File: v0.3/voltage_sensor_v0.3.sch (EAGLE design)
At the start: 56 parts, among them IC1 AP2112K-3.3TRG1, J2 236-404_000-009_999-950, J3 MC000048, J9 RJ11-6, T1 ZMPT101B, T2 ZMPT101B, T3 ZMPT101B

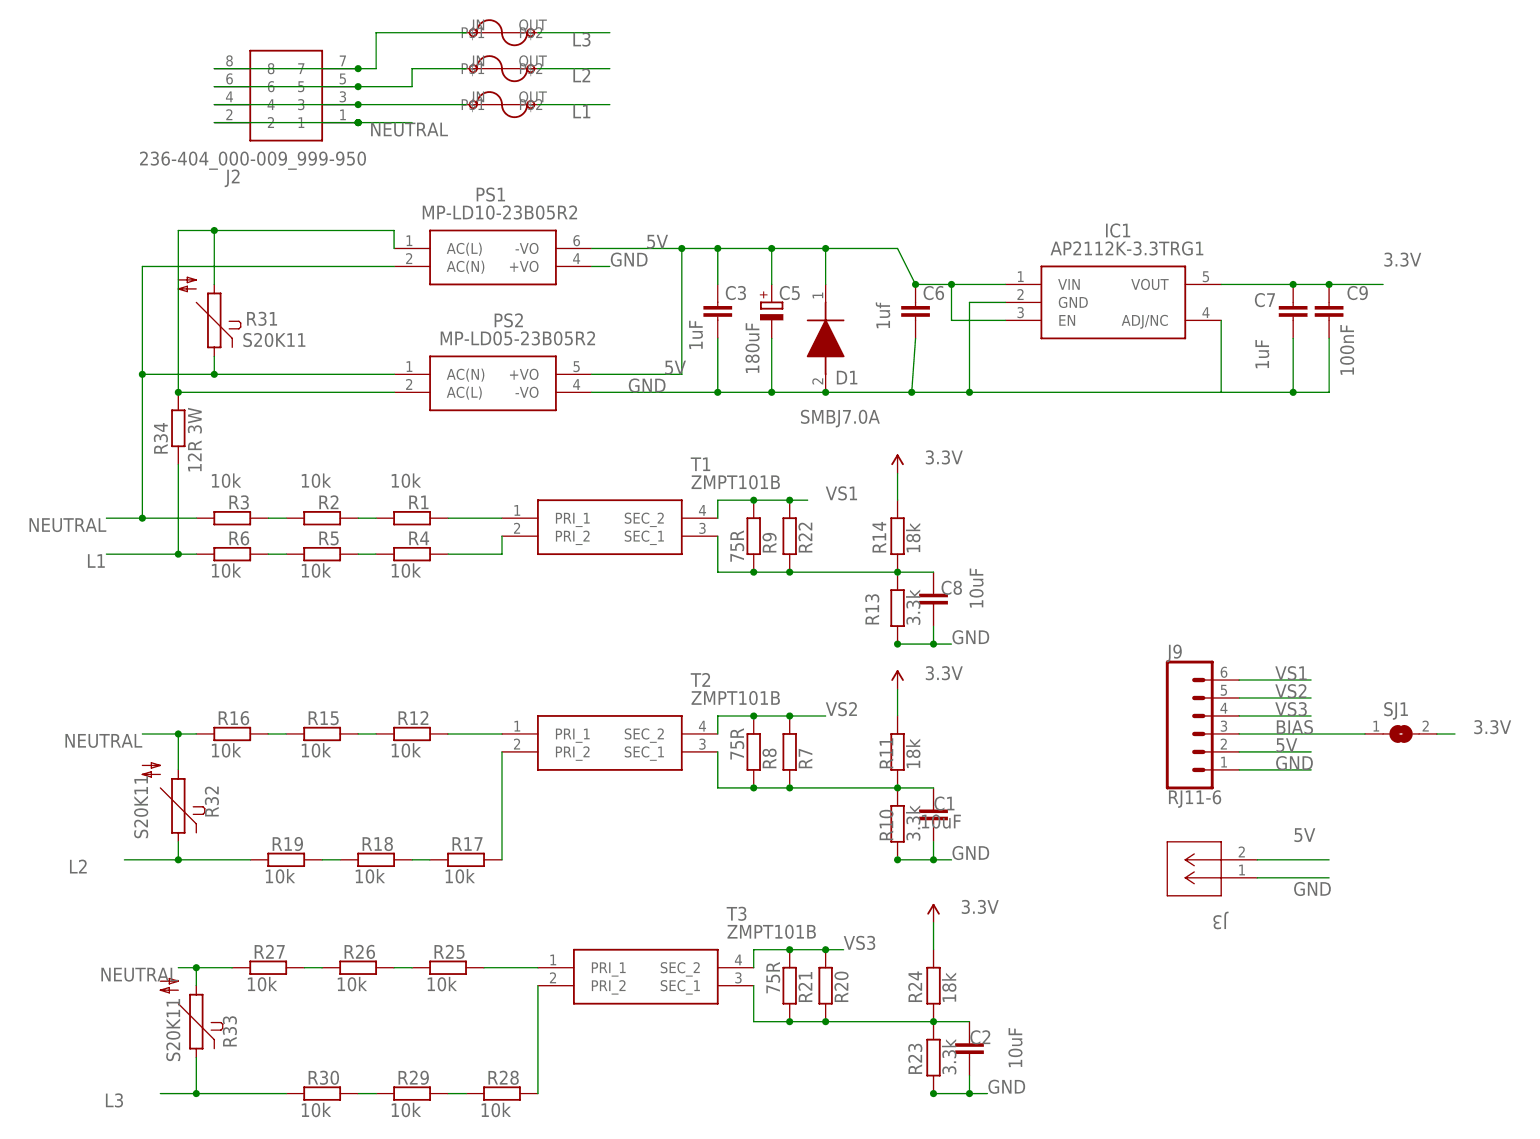
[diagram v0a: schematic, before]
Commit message: v0.3 changes
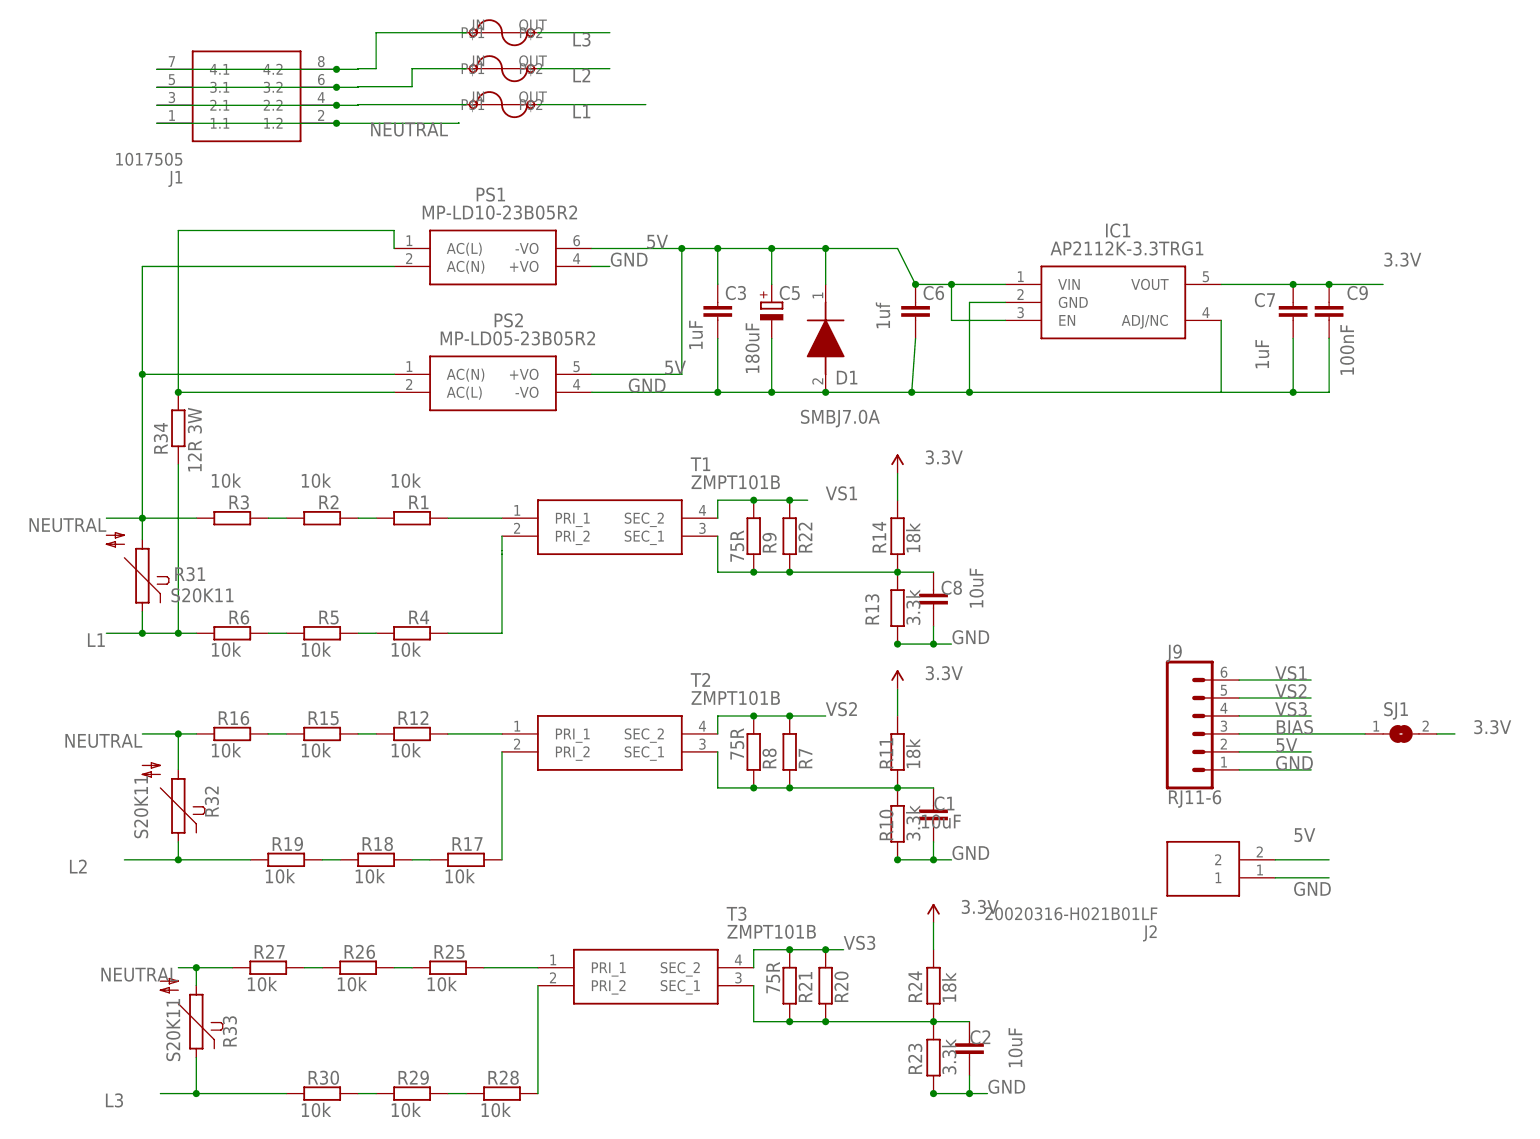
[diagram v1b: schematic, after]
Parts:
- removed J3: MC000048, 5mm-terminal:MC000048
- added J1: 1017505, 1017505:1017505
- J2: value 236-404_000-009_999-950 -> 20020316-H021B01LF; device 236-404_000-009_999-950:236-404_000-009_999-950 -> 20020316-H021B01LF:20020316-H021B01LF; ARROW_PART_NUMBER J2 -> (none)
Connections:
- net 5V: now also J2.2; no longer J3.2
- net GND: now also J2.1; no longer J3.1
- net L1: now also R31.1
- net N$16: now also J1.4.1, J1.4.2; no longer J2.7, J2.8
- net N$17: no longer R31.2
- net N$7: now also J1.2.1, J1.2.2; no longer J2.3, J2.4
- net N$8: now also J1.3.1, J1.3.2; no longer J2.5, J2.6
- net NEUTRAL: now also J1.1.1, J1.1.2, R31.2; no longer J2.1, J2.2, R31.1
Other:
- moved on the sheet: R31, R4, R5, R6
